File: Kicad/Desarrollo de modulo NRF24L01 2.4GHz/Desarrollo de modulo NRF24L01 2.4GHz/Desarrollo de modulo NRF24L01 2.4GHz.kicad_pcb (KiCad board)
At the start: 2 copper layers, 21 parts, among them J1 Conn_01x08_Pin, U1 NRF24L01, Y1 16MHz

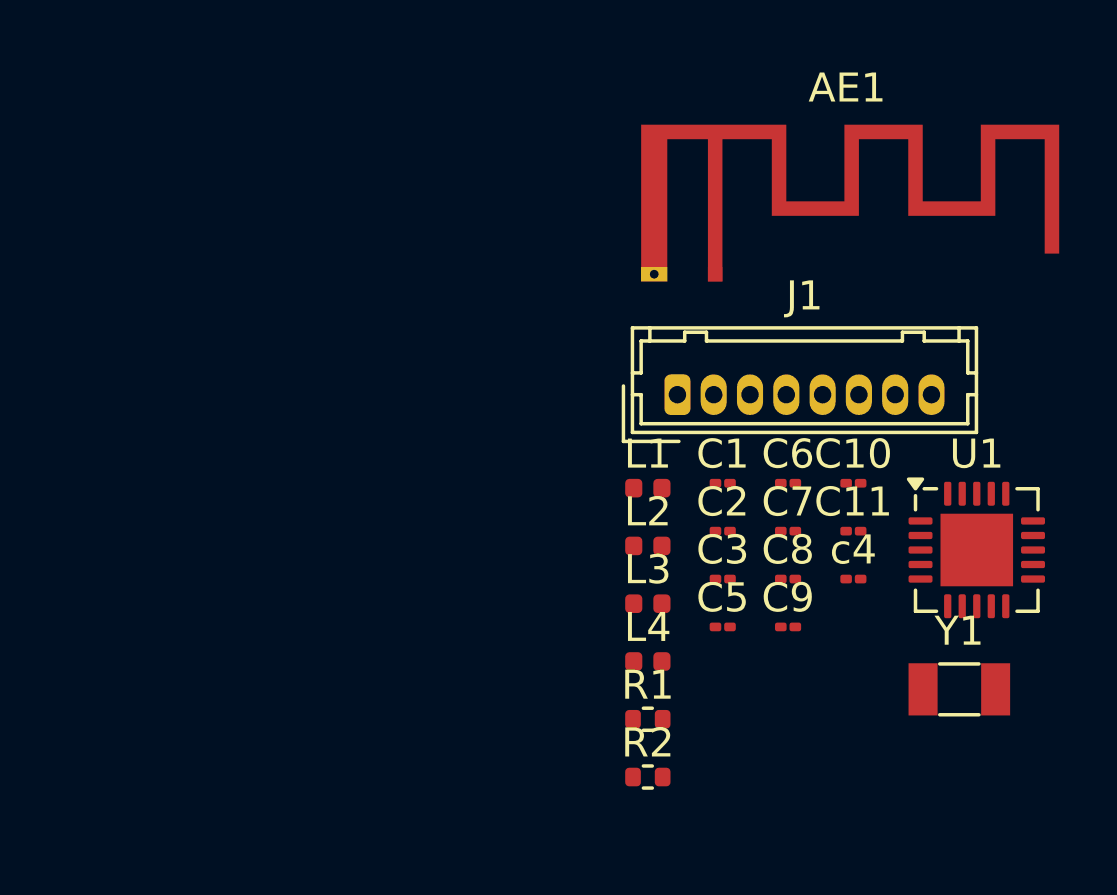
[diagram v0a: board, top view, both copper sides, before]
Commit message: Add files via upload
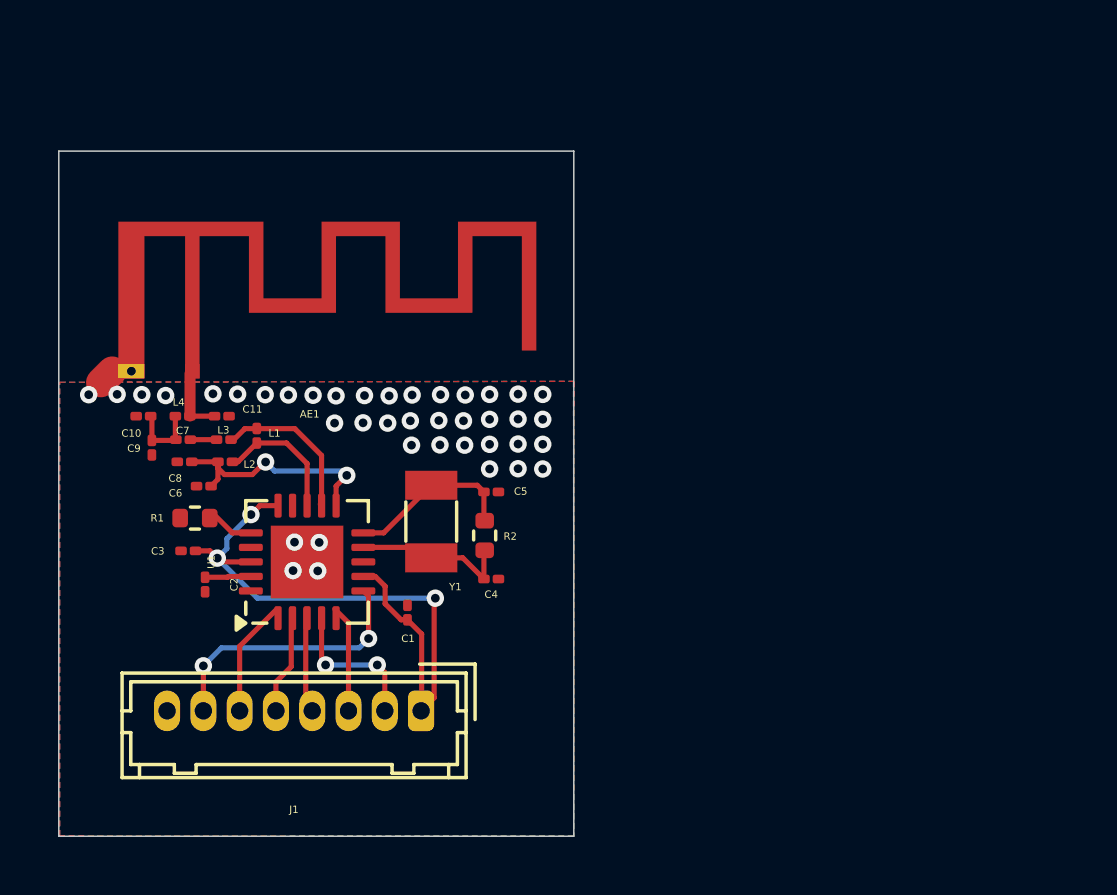
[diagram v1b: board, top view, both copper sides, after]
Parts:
- removed c4: 22p, Capacitor_SMD:C_01005_0402Metric
- added C4: 22p, Capacitor_SMD:C_01005_0402Metric, F.Cu at (112.1, 79.2)
- C1: value 33n -> 10n
- C2: value 10n -> 33n
- C7: value 1p5 -> 1n5
- L1, L4: footprint Inductor_SMD:L_0402_1005Metric -> Inductor_SMD:L_01005_0402Metric
- L2: value 3n9 -> 2n7; footprint Inductor_SMD:L_0402_1005Metric -> Inductor_SMD:L_01005_0402Metric
- L3: value 2n7 -> 3n9; footprint Inductor_SMD:L_0402_1005Metric -> Inductor_SMD:L_01005_0402Metric
- U1: value NRF24L01 -> nRF24L01P
- moved C10 24.6 mm to (100.1, 73.6), turned to 180 degrees
- moved U1 23.1 mm to (105.8, 78.6), turned to 90 degrees
- moved C9 22.8 mm to (100.4, 74.7), turned to -90 degrees
- moved C11 22.1 mm to (102.8, 73.6)
- moved C8 21.2 mm to (101.6, 75.2), turned to 180 degrees
- moved C7 21.1 mm to (101.5, 74.4), turned to 180 degrees
- moved C6 20.1 mm to (102.2, 76.0), turned to 180 degrees
- moved Y1 19.1 mm to (110.1, 77.2), turned to -90 degrees
- moved C3 18.4 mm to (101.7, 78.2), turned to 180 degrees
- moved AE1 18.3 mm to (101.8, 72.0)
- moved L4 18.1 mm to (101.5, 73.6)
- moved C2 17.9 mm to (102.3, 79.4), turned to -90 degrees
- moved R1 17.1 mm to (101.9, 77.1), turned to 180 degrees
- moved L3 15.7 mm to (102.9, 74.4), turned to 180 degrees
- moved L2 14.8 mm to (103.0, 75.2), turned to 180 degrees
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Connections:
- C1 pad 1: Net-(U1-DVDD) -> VDD
- C2 pad 1: VDD -> Net-(U1-DVDD)
- L2 pad 1: Net-(U1-ANT1) -> Net-(U1-ANT2)
- L2 pad 2: Net-(C7-Pad1) -> Net-(U1-VDD_PA)
- L3 pad 1: Net-(U1-VDD_PA) -> Net-(U1-ANT1)
- L3 pad 2: Net-(U1-ANT2) -> Net-(C7-Pad1)
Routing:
- net VDD: track 0.00 -> 23.1 mm, vias 0 -> 3
- net Net-(J1-Pin_7): track 0.00 -> 9.34 mm, vias 0 -> 2
- net Net-(U1-VDD_PA): track 0.00 -> 8.15 mm, vias 0 -> 2
- net Net-(U1-XC1): track 0.00 -> 5.93 mm
- net Net-(U1-XC2): track 0.00 -> 5.61 mm
- net Net-(U1-ANT1): track 0.00 -> 5.45 mm
- net Net-(J1-Pin_2): track 0.00 -> 5.14 mm, vias 0 -> 2
- net Net-(U1-ANT2): track 0.00 -> 4.58 mm
- net Net-(J1-Pin_6): track 0.00 -> 4.03 mm
- net Net-(J1-Pin_5): track 0.00 -> 3.72 mm
- net Net-(J1-Pin_3): track 0.00 -> 3.70 mm
- net Net-(J1-Pin_4): track 0.00 -> 3.59 mm
- net Net-(C10-Pad1): track 0.00 -> 2.51 mm
- net Net-(AE1-A): track 0.00 -> 2.29 mm
- net Net-(U1-IREF): track 0.00 -> 1.87 mm
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- added copper zone on B.Cu, net GND
- added copper zone on F.Cu, net GND
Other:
- board outline added: 17.7 x 23.6 mm
